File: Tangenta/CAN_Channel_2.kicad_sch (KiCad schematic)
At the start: 12 parts, among them J22 Conn_01x02_Pin, U20 ADM3053

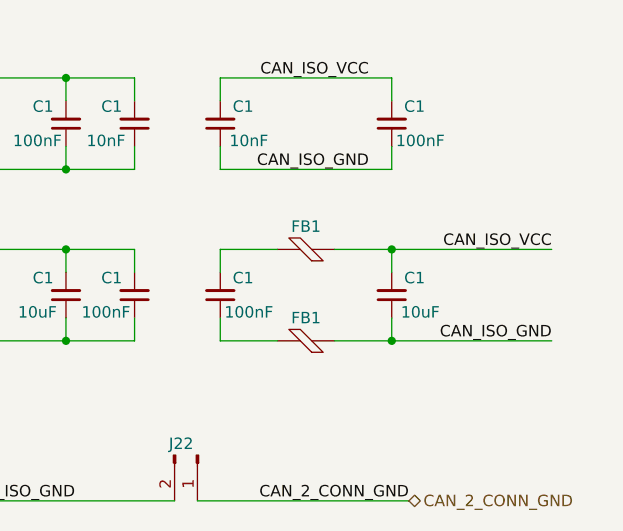
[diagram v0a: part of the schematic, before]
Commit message: CANbus - current progress.
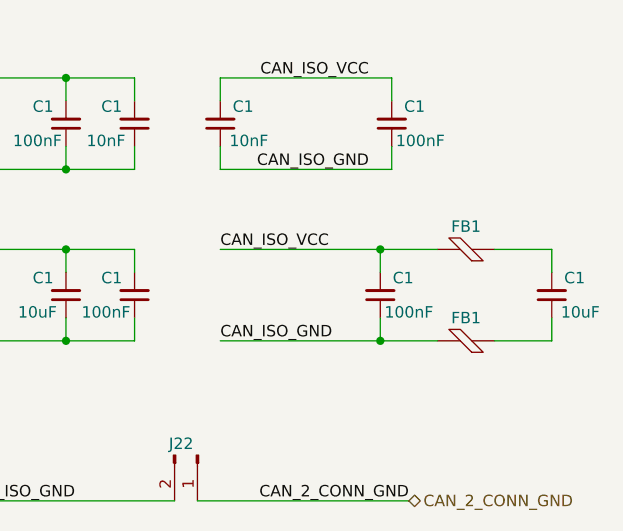
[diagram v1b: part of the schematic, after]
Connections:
- net CAN_ISO_GND: now also C1.1, FB1.1; no longer C1.1, FB1.2
- net CAN_ISO_VCC: now also C1.2, FB1.1; no longer C1.2, FB1.2
- new net: C1.2, FB1.2
- new net: C1.1, FB1.2
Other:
- moved on the sheet: C1, FB1
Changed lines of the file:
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@@
   (junction (at 151.765 80.01) (diameter 0) (color 0 0 0 0)
   )
-  (junction (at 160.655 140.97) (diameter 0) (color 0 0 0 0)
+  (junction (at 159.385 130.81) (diameter 0) (color 0 0 0 0)
   )
   (junction (at 124.46 121.92) (diameter 0) (color 0 0 0 0)
@@
   (junction (at 151.765 59.69) (diameter 0) (color 0 0 0 0)
   )
+  (junction (at 159.385 140.97) (diameter 0) (color 0 0 0 0)
+  )
   (junction (at 151.765 85.09) (diameter 0) (color 0 0 0 0)
   )
@@
   )
   (junction (at 122.555 85.09) (diameter 0) (color 0 0 0 0)
-  )
-  (junction (at 160.655 130.81) (diameter 0) (color 0 0 0 0)
   )
   (junction (at 122.555 80.01) (diameter 0) (color 0 0 0 0)
@@
     (stroke (width 0) (type default))
   )
-  (wire (pts (xy 160.655 140.97) (xy 178.435 140.97))
+  (wire (pts (xy 159.385 140.97) (xy 141.605 140.97))
     (stroke (width 0) (type default))
   )
@@
     (stroke (width 0) (type default))
   )
-  (wire (pts (xy 160.655 130.81) (xy 160.655 133.35))
+  (wire (pts (xy 178.435 130.81) (xy 178.435 133.35))
     (stroke (width 0) (type default))
   )
@@
     (stroke (width 0) (type default))
   )
-  (wire (pts (xy 160.655 138.43) (xy 160.655 140.97))
+  (wire (pts (xy 178.435 138.43) (xy 178.435 140.97))
     (stroke (width 0) (type default))
   )
@@
     (stroke (width 0) (type default))
   )
-  (wire (pts (xy 154.305 140.97) (xy 160.655 140.97))
+  (wire (pts (xy 172.085 140.97) (xy 178.435 140.97))
     (stroke (width 0) (type default))
   )
@@
     (stroke (width 0) (type default))
   )
-  (wire (pts (xy 154.305 130.81) (xy 160.655 130.81))
+  (wire (pts (xy 172.085 130.81) (xy 178.435 130.81))
     (stroke (width 0) (type default))
   )
@@
     (stroke (width 0) (type default))
   )
-  (wire (pts (xy 160.655 130.81) (xy 178.435 130.81))
+  (wire (pts (xy 159.385 130.81) (xy 141.605 130.81))
     (stroke (width 0) (type default))
   )
@@
     (stroke (width 0) (type default))
   )
-  (wire (pts (xy 141.605 130.81) (xy 141.605 133.35))
+  (wire (pts (xy 159.385 130.81) (xy 159.385 133.35))
     (stroke (width 0) (type default))
   )
@@
     (stroke (width 0) (type default))
   )
-  (wire (pts (xy 141.605 130.81) (xy 147.955 130.81))
+  (wire (pts (xy 159.385 130.81) (xy 165.735 130.81))
     (stroke (width 0) (type default))
   )
@@
     (stroke (width 0) (type default))
   )
-  (wire (pts (xy 141.605 140.97) (xy 147.955 140.97))
+  (wire (pts (xy 159.385 140.97) (xy 165.735 140.97))
     (stroke (width 0) (type default))
   )
@@
     (stroke (width 0) (type default))
   )
-  (wire (pts (xy 141.605 138.43) (xy 141.605 140.97))
+  (wire (pts (xy 159.385 138.43) (xy 159.385 140.97))
     (stroke (width 0) (type default))
   )
@@
     (effects (font (size 1.27 1.27)) (justify left bottom))
   )
-  (label "CAN_ISO_VCC" (at 178.435 130.81 180) (fields_autoplaced)
-    (effects (font (size 1.27 1.27)) (justify right bottom))
+  (label "CAN_ISO_VCC" (at 141.605 130.81 0) (fields_autoplaced)
+    (effects (font (size 1.27 1.27)) (justify left bottom))
   )
   (label "CAN_2_TX" (at 113.03 69.85 0) (fields_autoplaced)
@@
     (effects (font (size 1.27 1.27)) (justify right bottom))
   )
-  (label "CAN_ISO_GND" (at 178.435 140.97 180) (fields_autoplaced)
-    (effects (font (size 1.27 1.27)) (justify right bottom))
+  (label "CAN_ISO_GND" (at 141.605 140.97 0) (fields_autoplaced)
+    (effects (font (size 1.27 1.27)) (justify left bottom))
   )
   (label "CAN_ISO_GND" (at 158.115 121.92 180) (fields_autoplaced)
@@
     )
   )
-  (symbol (lib_id "Device:C_Small") (at 141.605 135.89 0) (mirror x) (unit 1)
-    (in_bom yes) (on_board yes) (dnp no)
-    (property "Reference" "C1" (at 144.1451 133.9849 0)
-      (effects (font (size 1.27 1.27)))
-    )
-    (property "Value" "100nF" (at 144.78 137.795 0)
-      (effects (font (size 1.27 1.27)))
-    )
-    (property "Footprint" "Capacitor_SMD:C_0402_1005Metric" (at 141.605 135.89 0)
-      (effects (font (size 1.27 1.27)) hide)
-    )
-    (property "Datasheet" "~" (at 141.605 135.89 0)
+  (symbol (lib_id "Device:C_Small") (at 159.385 135.89 0) (mirror x) (unit 1)
+    (in_bom yes) (on_board yes) (dnp no)
+    (property "Reference" "C1" (at 161.9251 133.9849 0)
+      (effects (font (size 1.27 1.27)))
+    )
+    (property "Value" "100nF" (at 162.56 137.795 0)
+      (effects (font (size 1.27 1.27)))
+    )
+    (property "Footprint" "Capacitor_SMD:C_0402_1005Metric" (at 159.385 135.89 0)
+      (effects (font (size 1.27 1.27)) hide)
+    )
+    (property "Datasheet" "~" (at 159.385 135.89 0)
       (effects (font (size 1.27 1.27)) hide)
     )
@@
     )
   )
-  (symbol (lib_id "Ferrite_Bead_100:GZ2012D101TF") (at 151.13 130.81 0) (unit 1)
-    (in_bom yes) (on_board yes) (dnp no)
-    (property "Reference" "FB1" (at 151.13 128.27 0)
-      (effects (font (size 1.27 1.27)))
-    )
-    (property "Value" "GZ2012D101TF" (at 151.13 127 0)
-      (effects (font (size 1.27 1.27)) hide)
-    )
-    (property "Footprint" "Ferrite_Bead_100:Ferrite_Bead_100" (at 163.703 140.843 0)
+  (symbol (lib_id "Ferrite_Bead_100:GZ2012D101TF") (at 168.91 130.81 0) (unit 1)
+    (in_bom yes) (on_board yes) (dnp no)
+    (property "Reference" "FB1" (at 168.91 128.27 0)
+      (effects (font (size 1.27 1.27)))
+    )
+    (property "Value" "GZ2012D101TF" (at 168.91 127 0)
+      (effects (font (size 1.27 1.27)) hide)
+    )
+    (property "Footprint" "Ferrite_Bead_100:Ferrite_Bead_100" (at 181.483 140.843 0)
       (effects (font (size 1.27 1.27) italic) hide)
     )
-    (property "Datasheet" "https://item.szlcsc.com/344132.html" (at 146.939 138.557 0)
+    (property "Datasheet" "https://item.szlcsc.com/344132.html" (at 164.719 138.557 0)
       (effects (font (size 1.27 1.27)) (justify left) hide)
     )
-    (property "LCSC" "C1015" (at 149.987 134.239 0)
+    (property "LCSC" "C1015" (at 167.767 134.239 0)
       (effects (font (size 1.27 1.27)) hide)
     )
@@
     )
   )
-  (symbol (lib_id "Ferrite_Bead_100:GZ2012D101TF") (at 151.13 140.97 0) (unit 1)
-    (in_bom yes) (on_board yes) (dnp no)
-    (property "Reference" "FB1" (at 151.13 138.43 0)
-      (effects (font (size 1.27 1.27)))
-    )
-    (property "Value" "GZ2012D101TF" (at 151.13 137.16 0)
-      (effects (font (size 1.27 1.27)) hide)
-    )
-    (property "Footprint" "Ferrite_Bead_100:Ferrite_Bead_100" (at 163.703 151.003 0)
+  (symbol (lib_id "Ferrite_Bead_100:GZ2012D101TF") (at 168.91 140.97 0) (unit 1)
+    (in_bom yes) (on_board yes) (dnp no)
+    (property "Reference" "FB1" (at 168.91 138.43 0)
+      (effects (font (size 1.27 1.27)))
+    )
+    (property "Value" "GZ2012D101TF" (at 168.91 137.16 0)
+      (effects (font (size 1.27 1.27)) hide)
+    )
+    (property "Footprint" "Ferrite_Bead_100:Ferrite_Bead_100" (at 181.483 151.003 0)
       (effects (font (size 1.27 1.27) italic) hide)
     )
-    (property "Datasheet" "https://item.szlcsc.com/344132.html" (at 146.939 148.717 0)
+    (property "Datasheet" "https://item.szlcsc.com/344132.html" (at 164.719 148.717 0)
       (effects (font (size 1.27 1.27)) (justify left) hide)
     )
-    (property "LCSC" "C1015" (at 149.987 144.399 0)
+    (property "LCSC" "C1015" (at 167.767 144.399 0)
       (effects (font (size 1.27 1.27)) hide)
     )
@@
     )
   )
-  (symbol (lib_id "Device:C_Small") (at 160.655 135.89 0) (mirror x) (unit 1)
-    (in_bom yes) (on_board yes) (dnp no)
-    (property "Reference" "C1" (at 163.1951 133.9849 0)
-      (effects (font (size 1.27 1.27)))
-    )
-    (property "Value" "10uF" (at 163.83 137.795 0)
-      (effects (font (size 1.27 1.27)))
-    )
-    (property "Footprint" "Capacitor_SMD:C_0402_1005Metric" (at 160.655 135.89 0)
-      (effects (font (size 1.27 1.27)) hide)
-    )
-    (property "Datasheet" "~" (at 160.655 135.89 0)
-      (effects (font (size 1.27 1.27)) hide)
-    )
+  (symbol (lib_id "Device:C_Small") (at 178.435 135.89 0) (mirror x) (unit 1)
+    (in_bom yes) (on_board yes) (dnp no)
+    (property "Reference" "C1" (at 180.9751 133.9849 0)
+      (effects (font (size 1.27 1.27)))
+    )
+    (property "Value" "10uF" (at 181.61 137.795 0)
+      (effects (font (size 1.27 1.27)))
+    )
+    (property "Footprint" "Capacitor_SMD:C_0402_1005Metric" (at 178.435 135.89 0)
+      (effects (font (size 1.27 1.27)) hide)
+    )
+    (property "Datasheet" "~" (at 178.435 135.89 0)
+      (effects (font (size 1.27 1.27)) hide)
+    )
